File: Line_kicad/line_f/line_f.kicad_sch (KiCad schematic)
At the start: 16 parts, among them M2 Motor_DC, M3 Motor_DC, SW1 SW_SPST, SW2 SW_SPDT, SW3 SW_Push, SW4 SW_Push, U1 TB6612FNG_LINE, m1 BLACKPILL

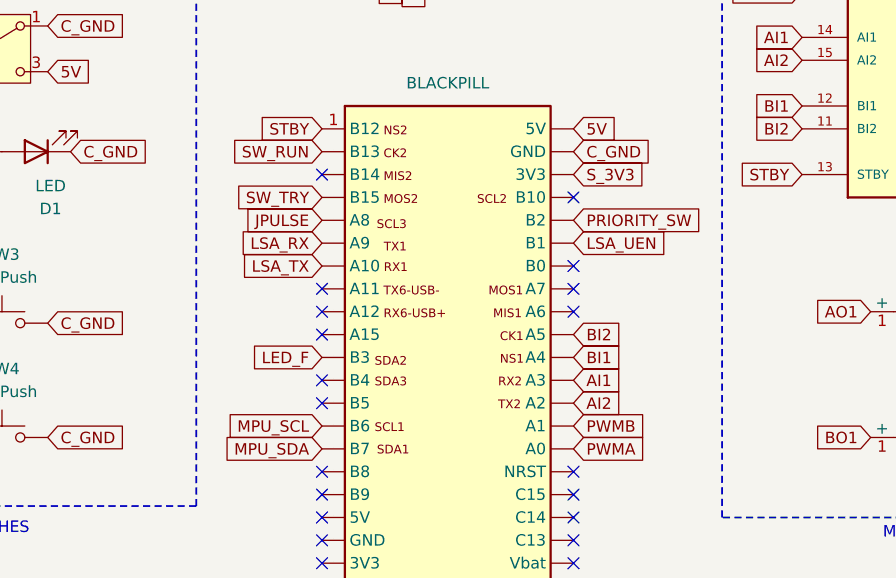
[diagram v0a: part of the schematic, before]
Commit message: 2#
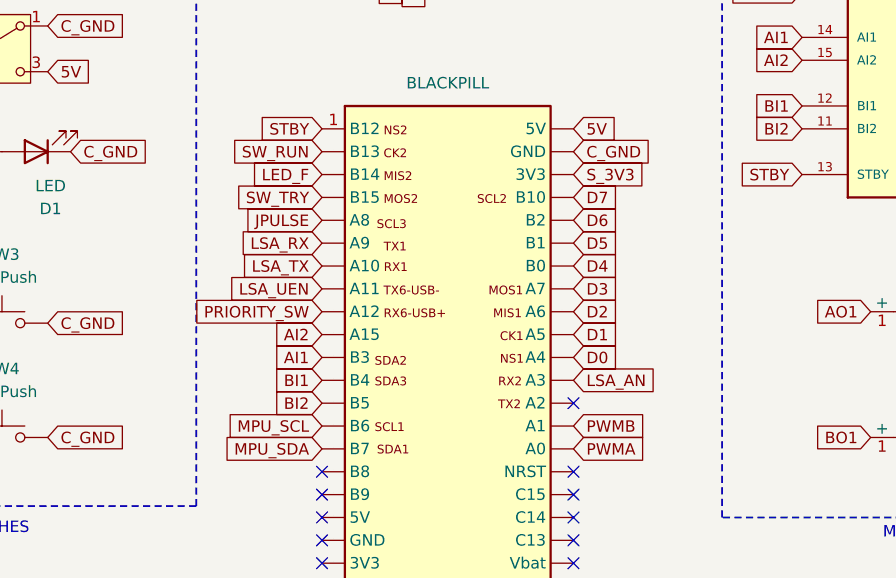
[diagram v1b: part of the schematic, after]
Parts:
- BUCK1: footprint TerminalBlock_Phoenix:TerminalBlock_Phoenix_PT-1,5-4-5.0-H_1x04_P5.00mm_Horizontal -> LINE_F_FOOT_LIB:BUCK_SMD
- D1: footprint LED_THT:LED_D1.8mm_W1.8mm_H2.4mm_Horizontal_O3.81mm_Z8.2mm -> LINE_F_FOOT_LIB:LED_LINE
- LSA_ANALOG1: footprint (none) -> LINE_F_FOOT_LIB:LSA_ANALOG
- LSA_DIGITAL1: footprint (none) -> LINE_F_FOOT_LIB:LSA_DIGITAL
- LSA_UART1: footprint (none) -> LINE_F_FOOT_LIB:LSA_UART
- M2: footprint Connector_JST:JST_XH_S2B-XH-A-1_1x02_P2.50mm_Horizontal -> LINE_F_FOOT_LIB:connector_motor
- M3: footprint Connector_JST:JST_XH_B2B-XH-A_1x02_P2.50mm_Vertical -> LINE_F_FOOT_LIB:connector_motor
- MPU1: footprint (none) -> LINE_F_FOOT_LIB:MPU6050_AR
- R1: footprint Resistor_THT:R_Axial_DIN0309_L9.0mm_D3.2mm_P2.54mm_Vertical -> LINE_F_FOOT_LIB:RESISTOR_LINE
- SW1: footprint Button_Switch_THT:SW_MEC_5GTH9 -> LINE_F_FOOT_LIB:BATTERY_SW_FOOT
- SW2: footprint Button_Switch_THT:SW_Push_1P2T_Vertical_E-Switch_800UDP8P1A1M6 -> LINE_F_FOOT_LIB:SLIDE SW
- SW3, SW4: footprint Button_Switch_THT:SW_PUSH_6mm_H13mm -> LINE_F_FOOT_LIB:push_button
- U1: footprint ROB-14450:MODULE_ROB-14450 -> LINE_F_FOOT_LIB:TB6612FNG_LINE
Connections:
- net AI1: now also m1.11 (B3); no longer m1.32 (A3)
- net AI2: now also m1.10 (A15); no longer m1.33 (A2)
- net BI1: now also m1.12 (B4); no longer m1.31 (A4)
- net BI2: now also m1.13 (B5); no longer m1.30 (A5)
- net D0: now also m1.31 (A4)
- net D1: now also m1.30 (A5)
- net D2: now also m1.29 (A6)
- net D3: now also m1.28 (A7)
- net D4: now also m1.27 (B0)
- net D5: now also m1.26 (B1)
- net D6: now also m1.25 (B2)
- net D7: now also m1.24 (B10)
- net LED_F: now also m1.3 (B14); no longer m1.11 (B3)
- net LSA_AN: now also m1.32 (A3)
- net LSA_UEN: now also m1.8 (A11); no longer m1.26 (B1)
- net PRIORITY_SW: now also m1.9 (A12); no longer m1.25 (B2)
- no-connect marks 22 -> 13

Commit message: 3#
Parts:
- SW1: footprint LINE_F_FOOT_LIB:BATTERY_SW_FOOT -> LINE_F_FOOT_LIB:battery_sw
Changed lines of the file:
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@@
 			)
 		)
-		(property "Footprint" "LINE_F_FOOT_LIB:BATTERY_SW_FOOT"
+		(property "Footprint" "LINE_F_FOOT_LIB:battery_sw"
 			(at 82.55 109.22 0)
 			(effects

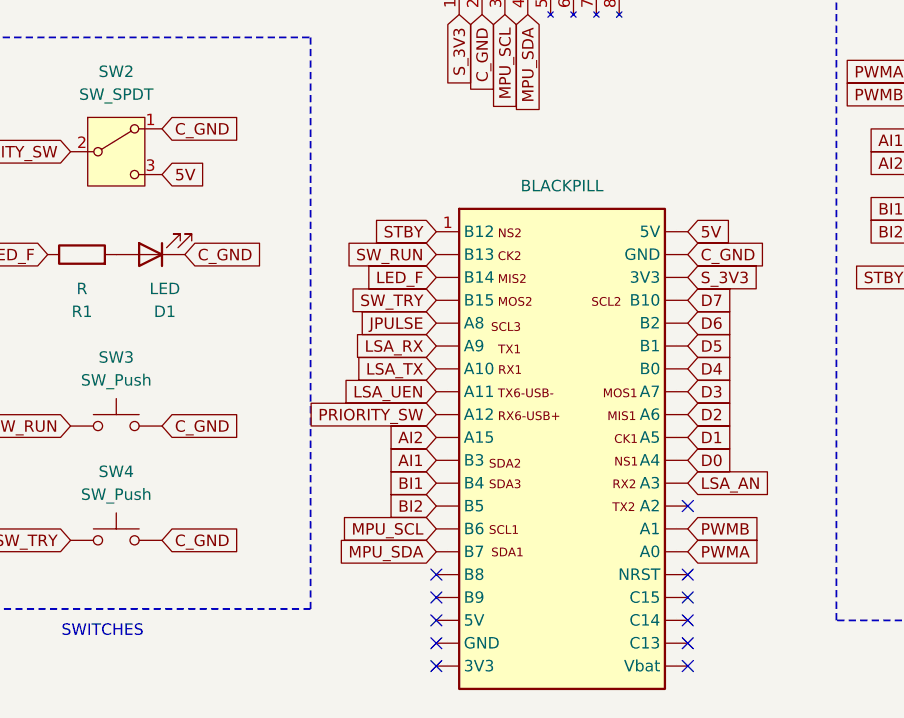
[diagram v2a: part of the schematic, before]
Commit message: 3#
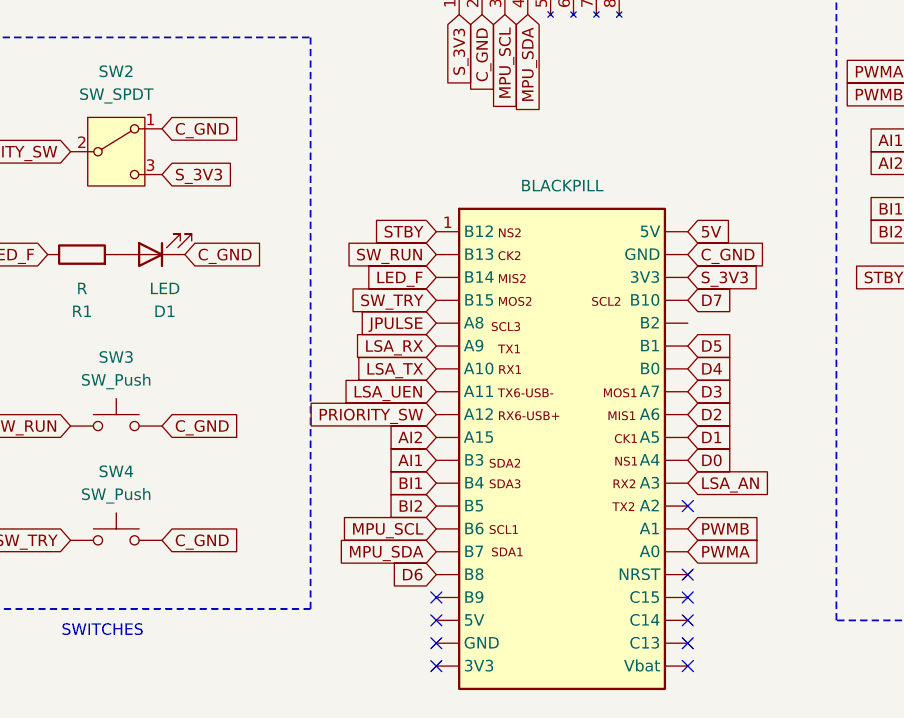
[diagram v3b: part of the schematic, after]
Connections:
- net 5V: no longer SW2.3 (C)
- net D6: now also m1.16 (B8); no longer m1.25 (B2)
- net S_3V3: now also SW2.3 (C)
- no-connect marks 13 -> 12
